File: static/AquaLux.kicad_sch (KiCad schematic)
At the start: 7 parts, among them Q1 NPN, U1 ESP32-S2

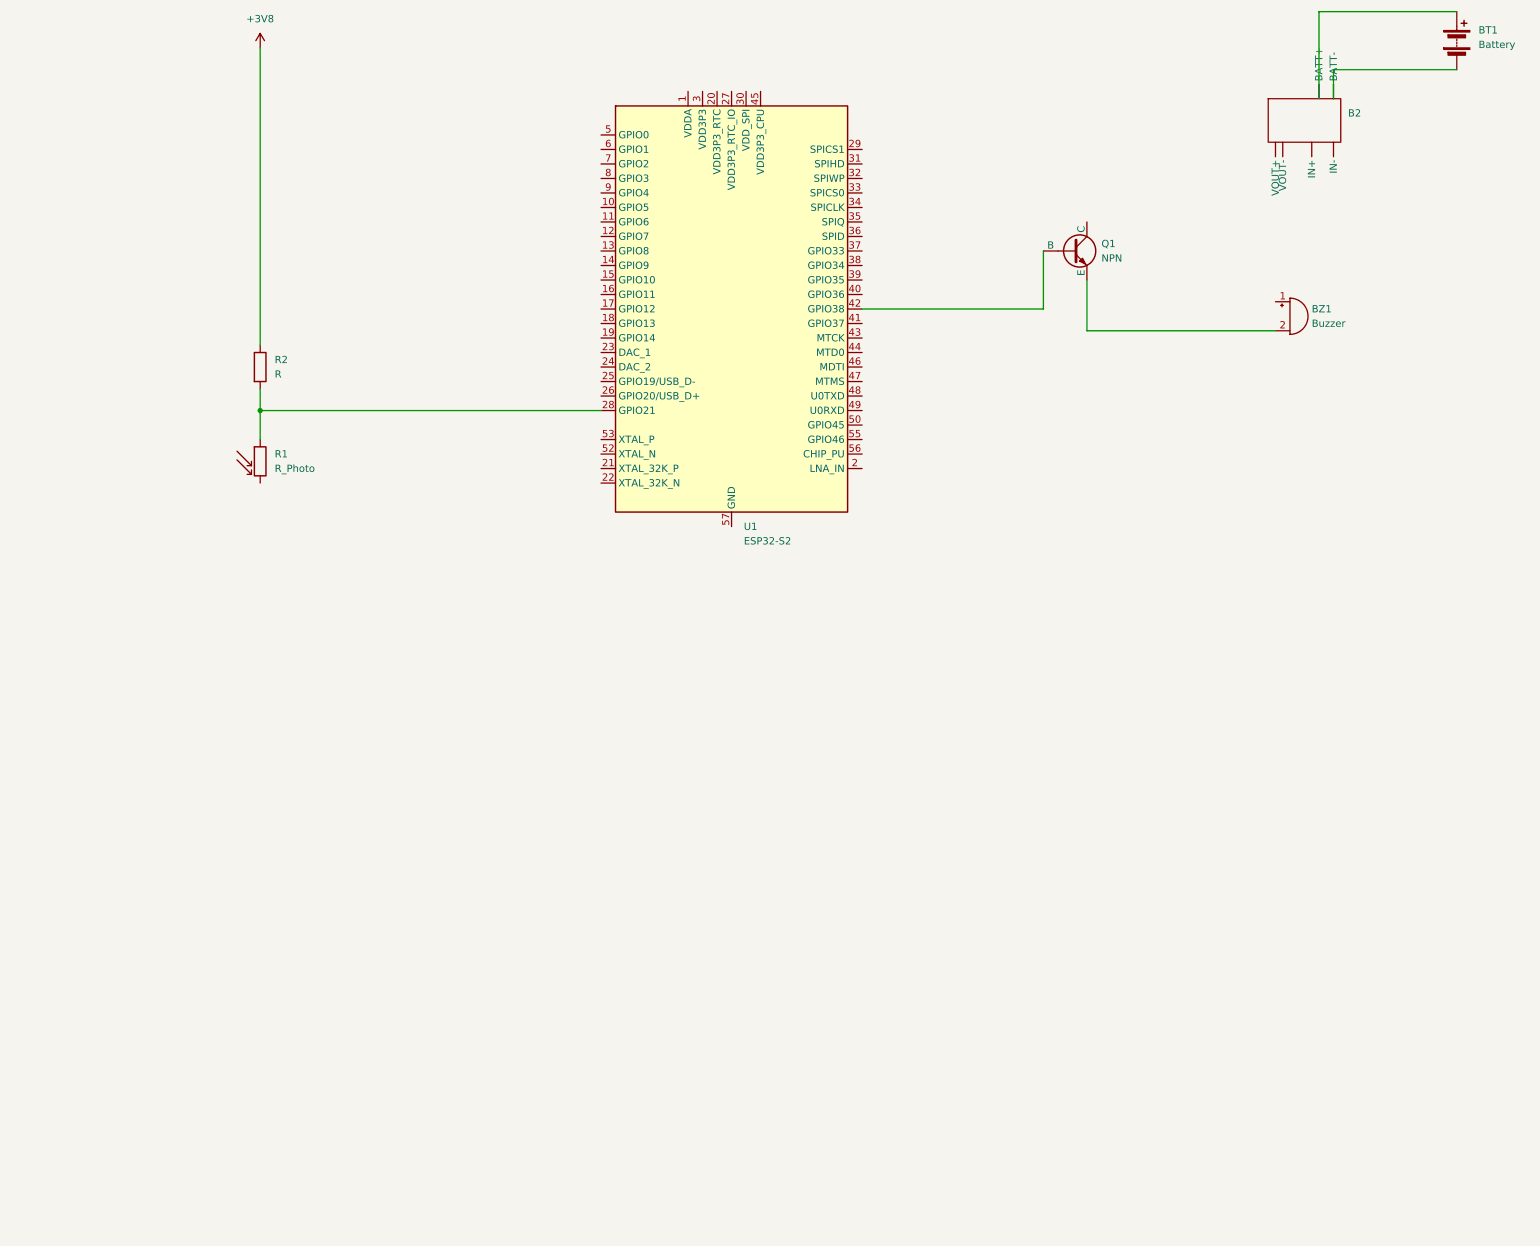
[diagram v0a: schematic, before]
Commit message: added kicad schematics properly.
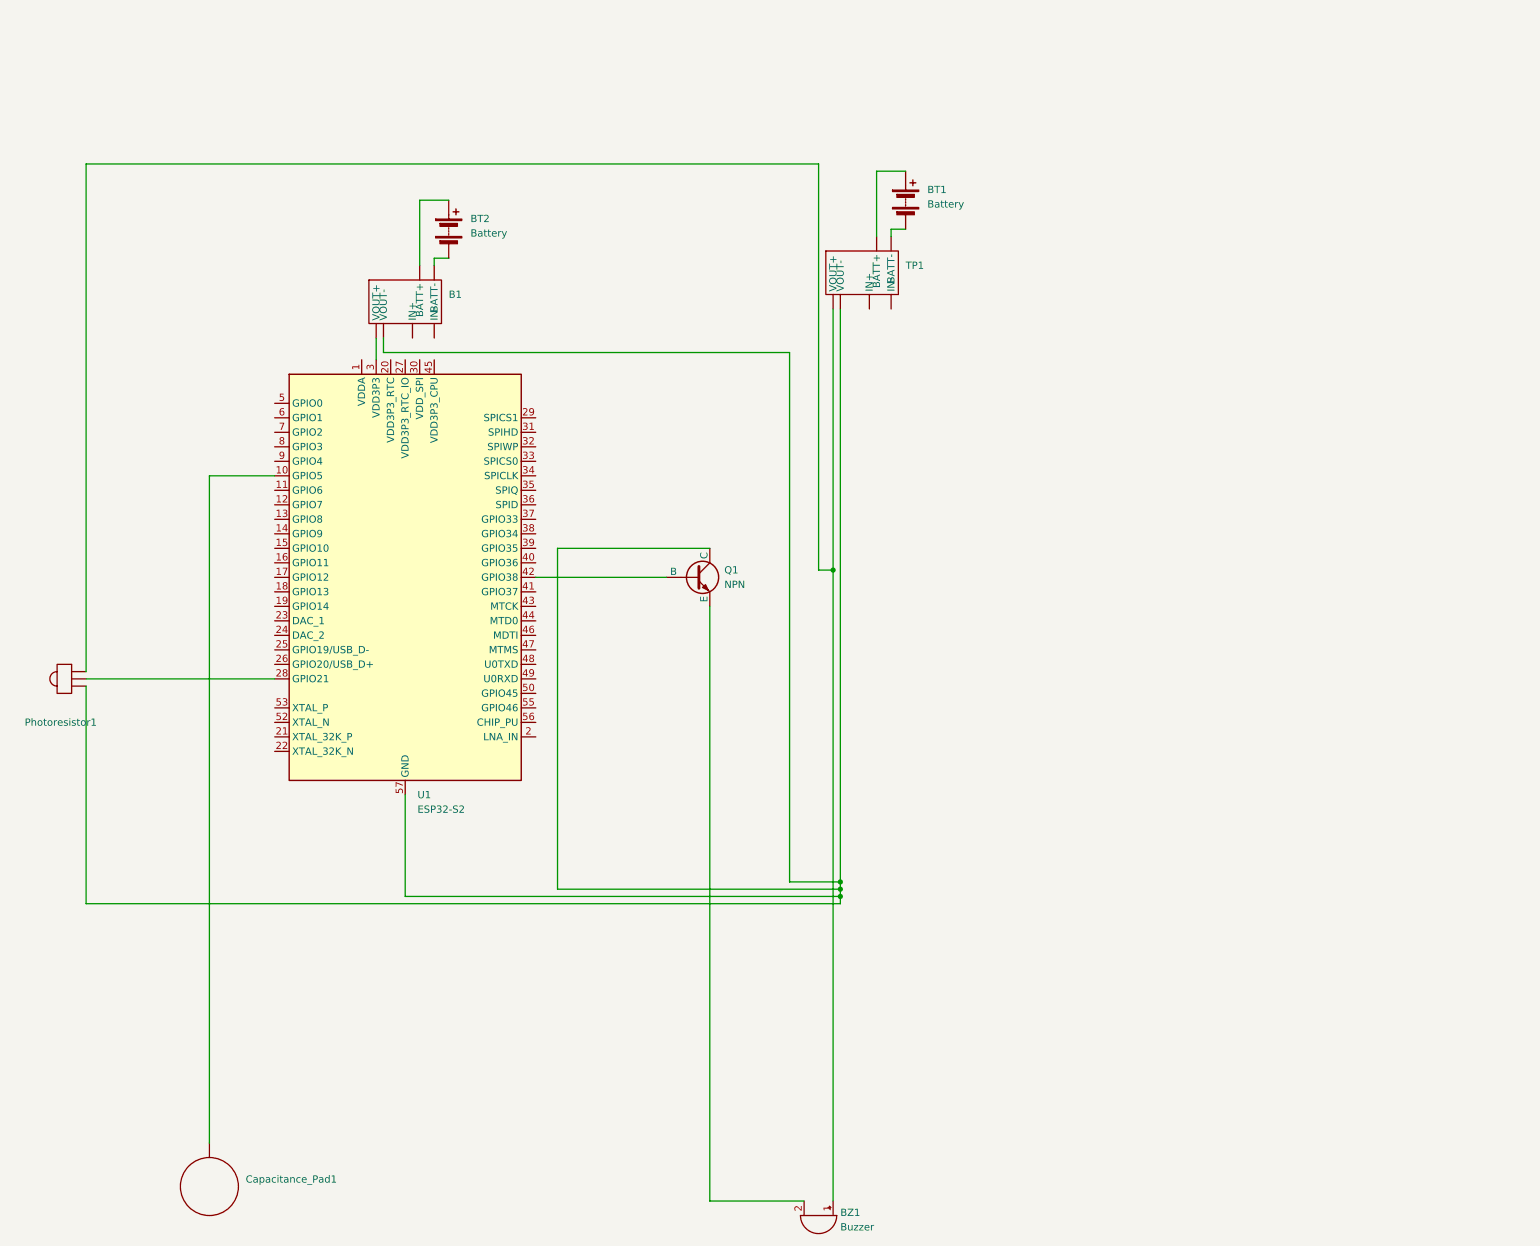
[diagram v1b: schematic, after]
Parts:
- removed B2: ~, symbol Custom_symbols:B5109
- removed R1: R_Photo, symbol Device:R_Photo
- removed R2: R, symbol Device:R
- added B1: ~, symbol Custom_symbols:B5109
- added BT2: Battery, symbol Device:Battery
- added Capacitance_Pad1: ~, symbol Custom_symbols:Capacitance_Pad
- added Photoresistor1: ~, symbol Custom_symbols:Photoresistor
- added TP1: ~, symbol Custom_symbols:TP4056
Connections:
- net at U1.28 (GPIO21): now also Photoresistor1. (GND)
- net at BT1.1 (+): now also TP1. (IN-)
- net at BT1.2 (-): now also TP1. (IN-)
- net at U1.10 (GPIO5): now also Capacitance_Pad1.
- net at U1.3 (VDD3P3), U1.4 (VDD3P3): now also B1. (IN-)
- net at U1.57 (GND): now also Q1.1 (C), B1. (IN-), Photoresistor1. (GND), TP1. (IN-)
- net at BZ1.1 (+): now also Photoresistor1. (GND), TP1. (IN-)
- new net: B1. (IN-), BT2.1 (+)
- new net: B1. (IN-), BT2.2 (-)
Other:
- company: (none) -> Adyansh
- title: (none) -> Aqualux circuit diagram
- moved on the sheet: BT1, BZ1, Q1, U1
